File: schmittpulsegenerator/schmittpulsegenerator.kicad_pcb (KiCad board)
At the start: 2 copper layers, 45.7 x 30.5 mm, 15 parts, among them J1 Conn_Coaxial, J2 Conn_01x02_Male, U1 74HC14

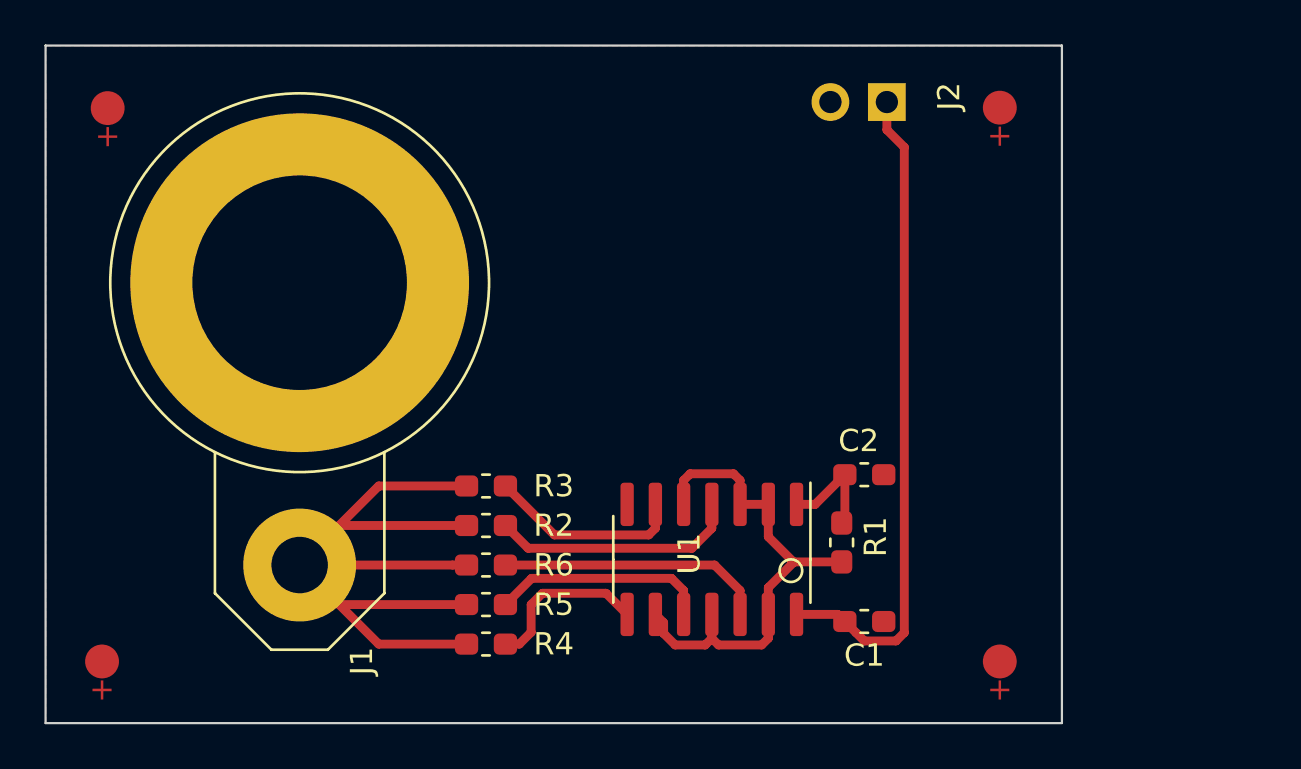
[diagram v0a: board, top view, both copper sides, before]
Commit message: stuff
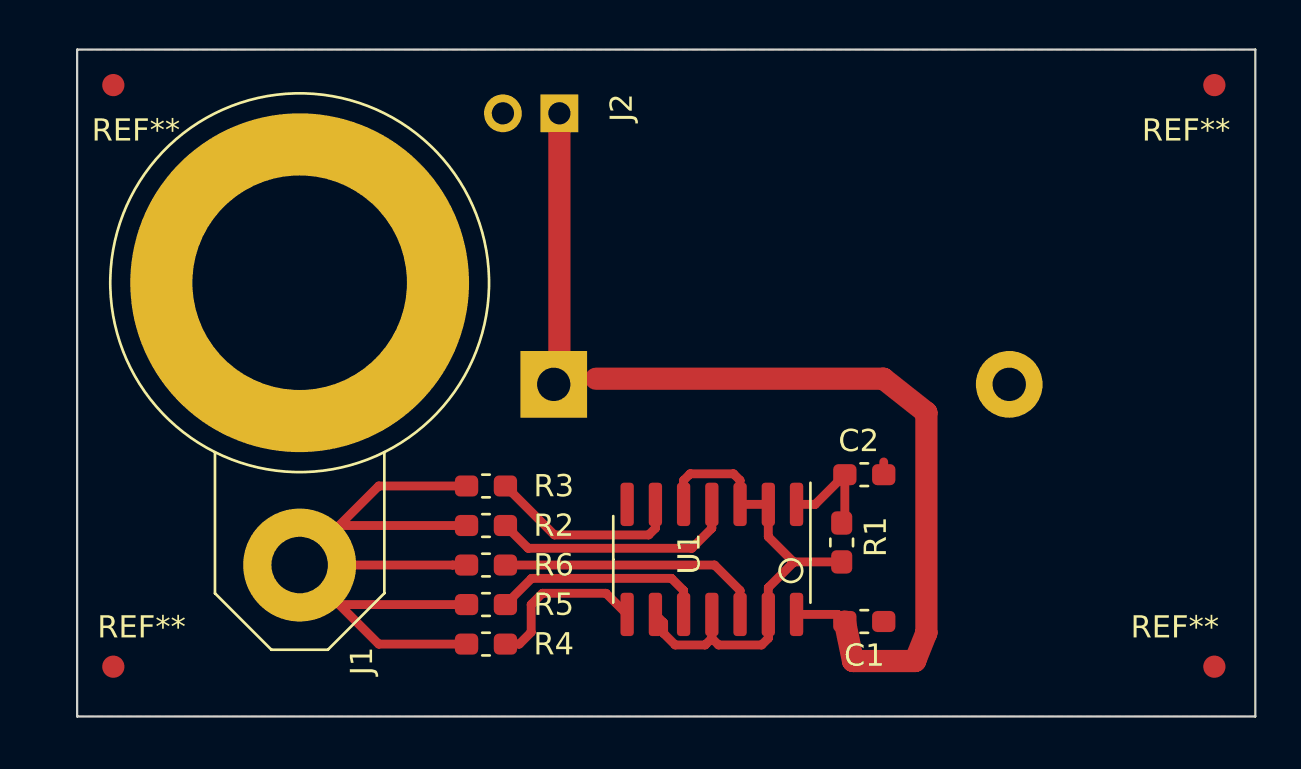
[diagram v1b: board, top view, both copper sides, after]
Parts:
- removed the REF** at (111.5, 112.8)
- removed the REF** at (71.1, 112.8)
- removed the REF** at (111.5, 87.9)
- removed the REF** at (71.4, 87.9)
- added BT1: Battery_Cell, Battery:Battery_Cell, B.Cu at (91.4, 99.1)
- added REF**: Fiducial_0.5mm_Mask1.5mm, kicad footprint libraries:Fiducial_0.5mm_Mask1.5mm, F.Cu at (71.6, 111.8)
- added REF**: Fiducial_0.5mm_Mask1.5mm, kicad footprint libraries:Fiducial_0.5mm_Mask1.5mm, F.Cu at (121.2, 111.8)
- added REF**: Fiducial_0.5mm_Mask1.5mm, kicad footprint libraries:Fiducial_0.5mm_Mask1.5mm, F.Cu at (121.2, 85.6)
- added REF**: Fiducial_0.5mm_Mask1.5mm, kicad footprint libraries:Fiducial_0.5mm_Mask1.5mm, F.Cu at (71.6, 85.6)
- moved J2 14.7 mm to (91.7, 86.9)
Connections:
- net +5V renamed +BATT
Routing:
- net +BATT: track 29.7 -> 48.2 mm
- net GND: track 0.00 -> 0.57 mm
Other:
- board size 45.7 x 30.5 mm -> 53 x 30 mm
